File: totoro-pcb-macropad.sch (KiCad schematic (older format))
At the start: 37 parts, among them J1 USB4085-GF-A_REVA, SW1 SW_PUSH, U1 ATMEGA32U4, X1 XTAL_GND

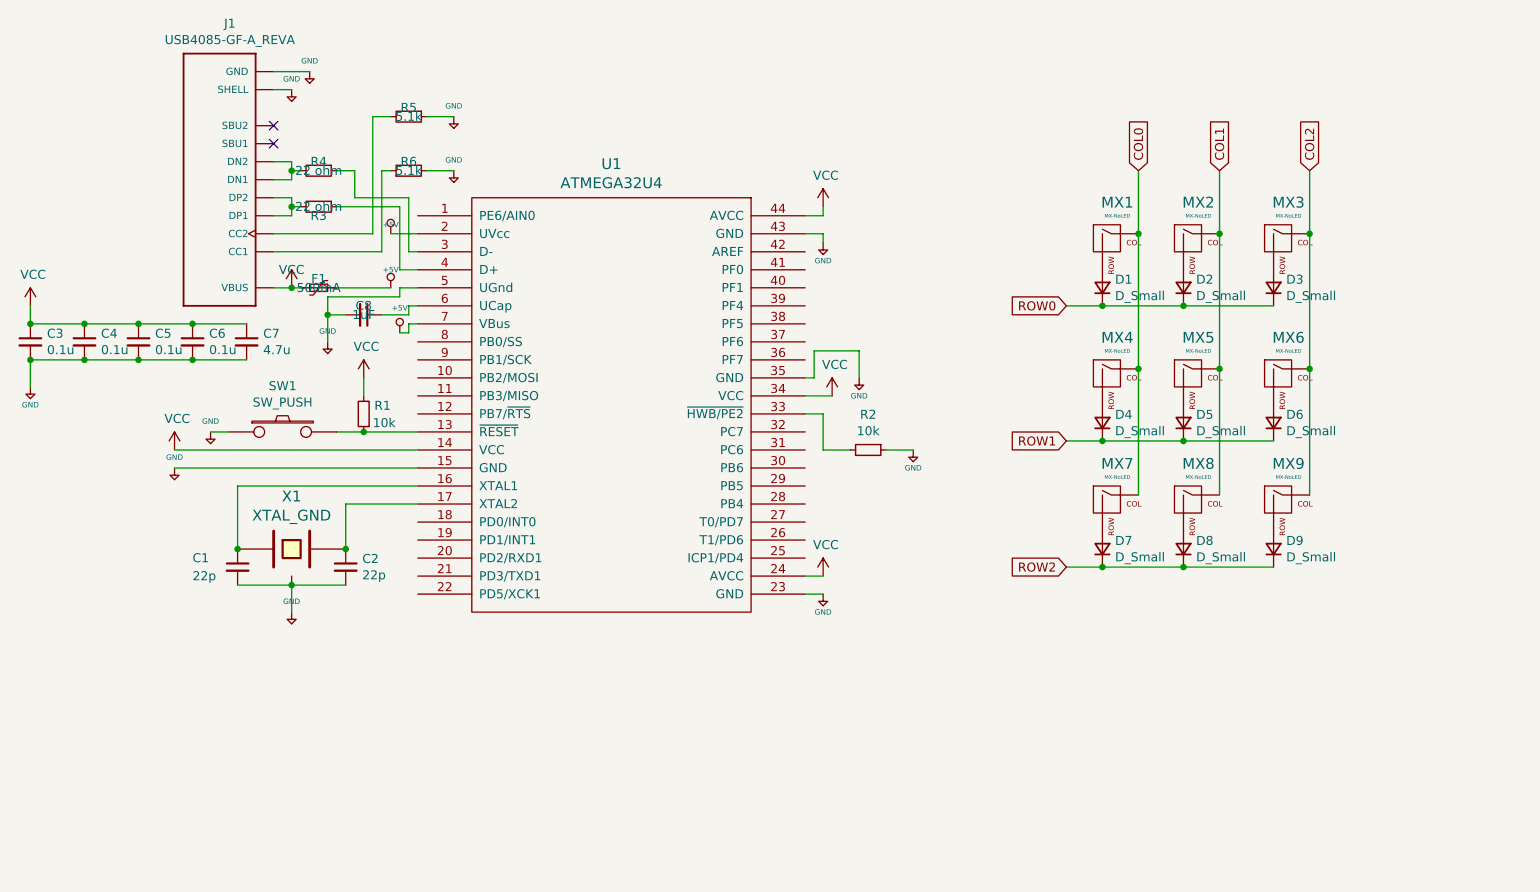
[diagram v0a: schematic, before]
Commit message: PCB layout
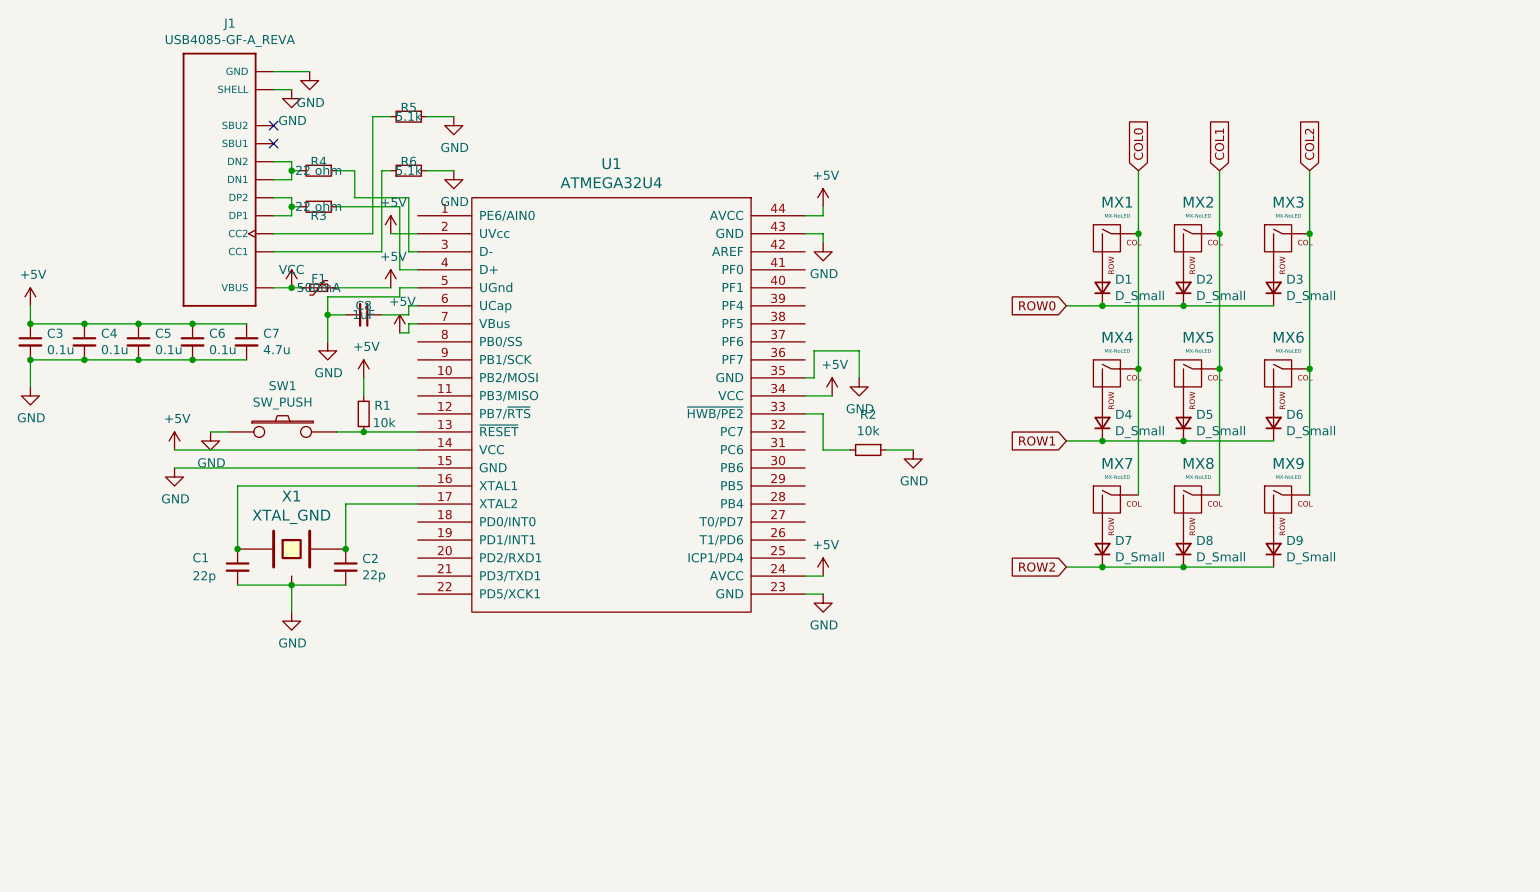
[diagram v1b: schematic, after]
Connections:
- net +5V: now also C3.1, C4.1, C5.1, C6.1, C7.1, R1.2, U1.14 (VCC), U1.24 (AVCC), U1.34 (VCC), U1.44 (AVCC); no longer C1.2, C2.2, C3.2, C4.2, C5.2, C6.2, C7.2, C8.2, J1.A1 (GND), J1.A12 (GND), J1.B1 (GND), J1.B12 (GND), J1.P1 (SHELL), J1.P2 (SHELL), J1.P3 (SHELL), J1.P4 (SHELL), R2.1, R5.1, R6.2, SW1.1, U1.15 (GND), U1.23 (GND), U1.35 (GND), U1.43 (GND), U1.5 (UGnd), X1.3
- net VCC: no longer C3.1, C4.1, C5.1, C6.1, C7.1, R1.2, U1.14 (VCC), U1.24 (AVCC), U1.34 (VCC), U1.44 (AVCC)
- new net GND: C1.2, C2.2, C3.2, C4.2, C5.2, C6.2, C7.2, C8.2, J1.A1 (GND), J1.A12 (GND), J1.B1 (GND), J1.B12 (GND), J1.P1 (SHELL), J1.P2 (SHELL), J1.P3 (SHELL), J1.P4 (SHELL), R2.1, R5.1, R6.2, SW1.1, U1.15 (GND), U1.23 (GND), U1.35 (GND), U1.43 (GND), U1.5 (UGnd), X1.3

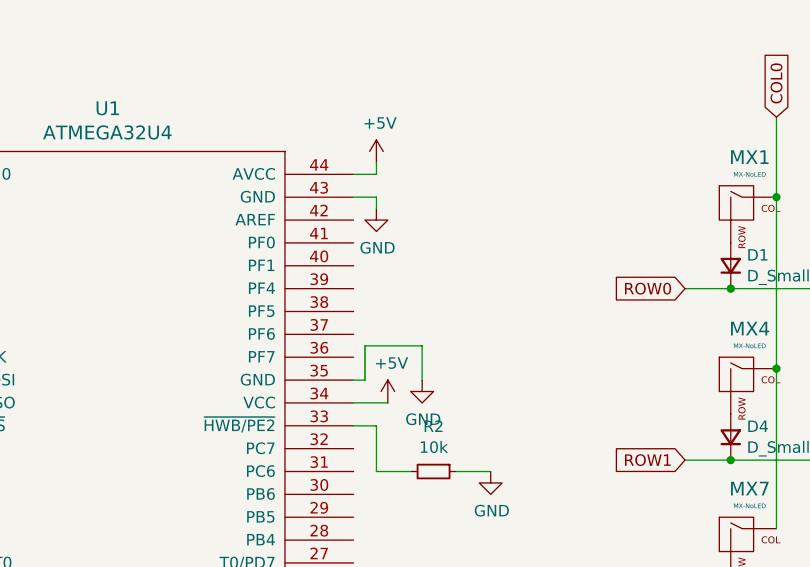
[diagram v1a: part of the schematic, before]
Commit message: Final commit
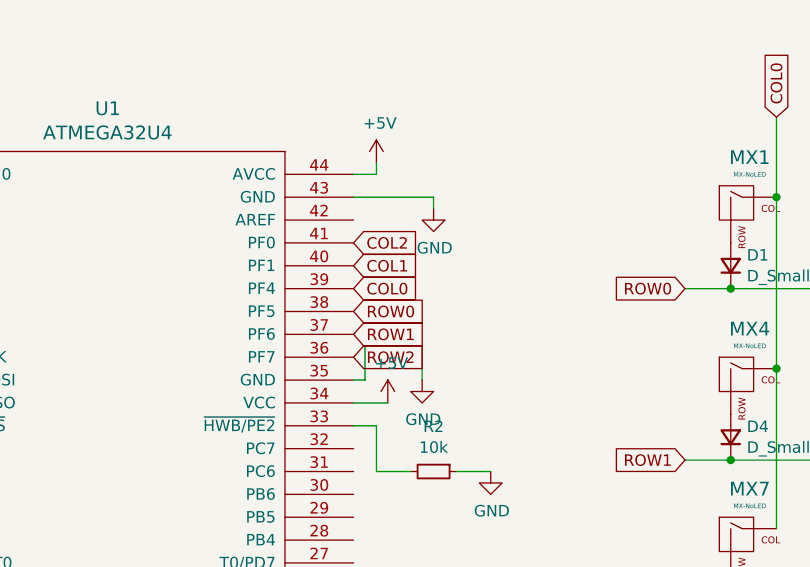
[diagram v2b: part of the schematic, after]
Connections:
- net COL0: now also U1.39 (PF4)
- net COL1: now also U1.40 (PF1)
- net COL2: now also U1.41 (PF0)
- net ROW0: now also U1.38 (PF5)
- net ROW1: now also U1.37 (PF6)
- net ROW2: now also U1.36 (PF7)
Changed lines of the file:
@@
 	2600 2250 2600 2400
-Wire Wire Line
-	5250 1800 5350 1800
-Wire Wire Line
-	5350 1800 5350 1850
 Wire Wire Line
 	5250 1700 5350 1700
@@
 L power:GND #PWR0105
 U 1 1 5F4F7593
-P 5350 1850
-F 0 "#PWR0105" H 5350 1600 50  0001 C CNN
-F 1 "GND" H 5355 1677 50  0000 C CNN
-F 2 "" H 5350 1850 50  0001 C CNN
-F 3 "" H 5350 1850 50  0001 C CNN
-	1    5350 1850
+P 5600 1850
+F 0 "#PWR0105" H 5600 1600 50  0001 C CNN
+F 1 "GND" H 5605 1677 50  0000 C CNN
+F 2 "" H 5600 1850 50  0001 C CNN
+F 3 "" H 5600 1850 50  0001 C CNN
+	1    5600 1850
 	1    0    0    -1
 $EndComp
@@
 	1    0    0    -1
 $EndComp
+Text GLabel 5250 2000 2    50   Input ~ 0
+COL2
+Wire Wire Line
+	5600 1800 5600 1850
+Wire Wire Line
+	5250 1800 5600 1800
+Text GLabel 5250 2100 2    50   Input ~ 0
+COL1
+Text GLabel 5250 2200 2    50   Input ~ 0
+COL0
+Text GLabel 5250 2300 2    50   Input ~ 0
+ROW0
+Text GLabel 5250 2400 2    50   Input ~ 0
+ROW1
+Text GLabel 5250 2500 2    50   Input ~ 0
+ROW2
 $EndSCHEMATC

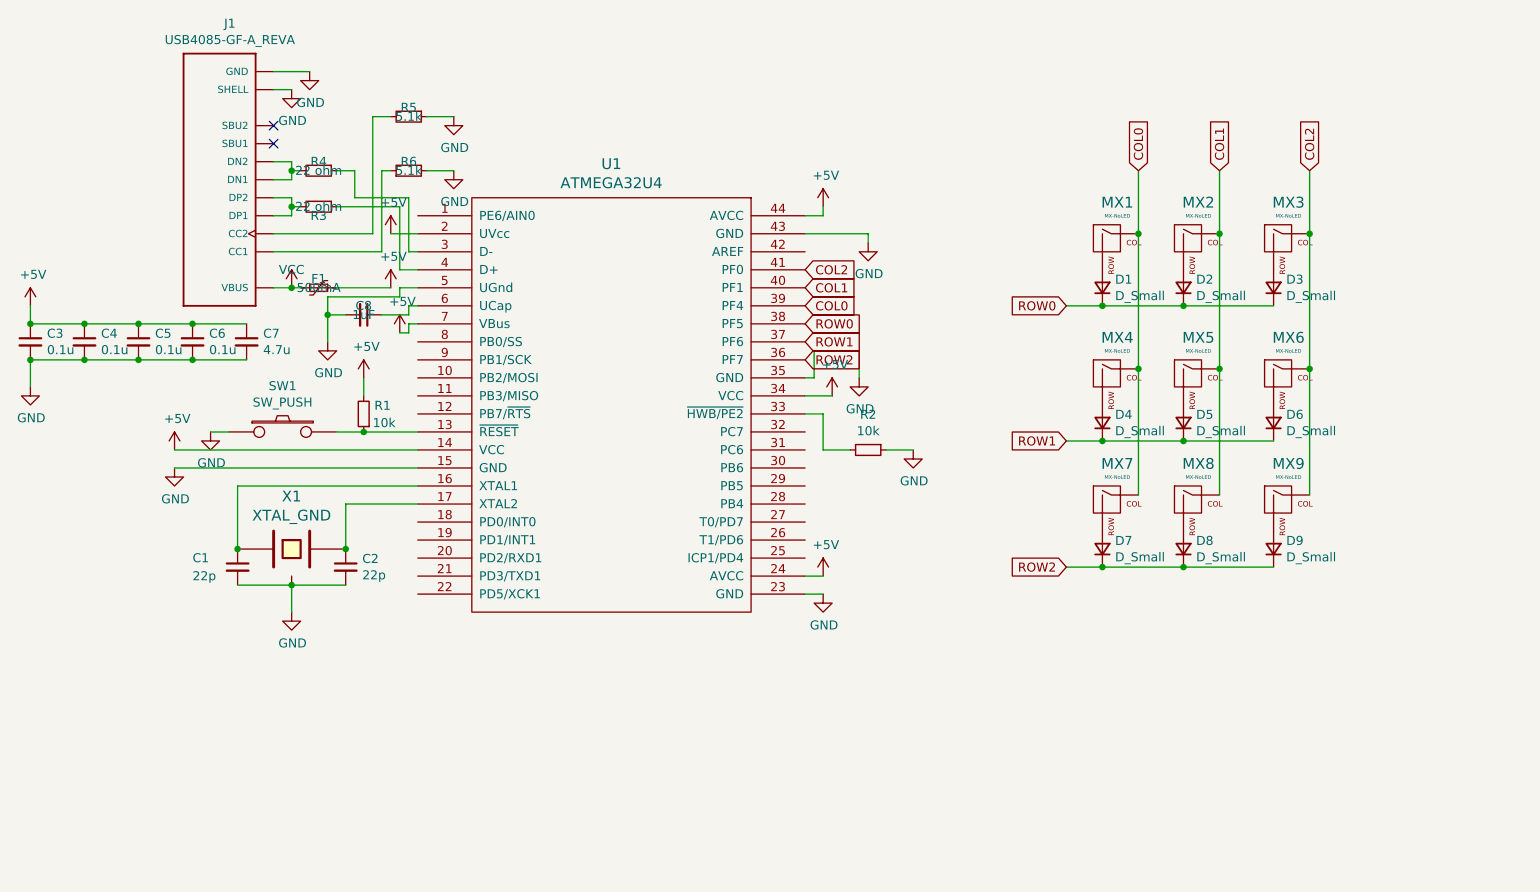
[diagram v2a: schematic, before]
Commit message: Probably fix crystal footprint, but i dont remember
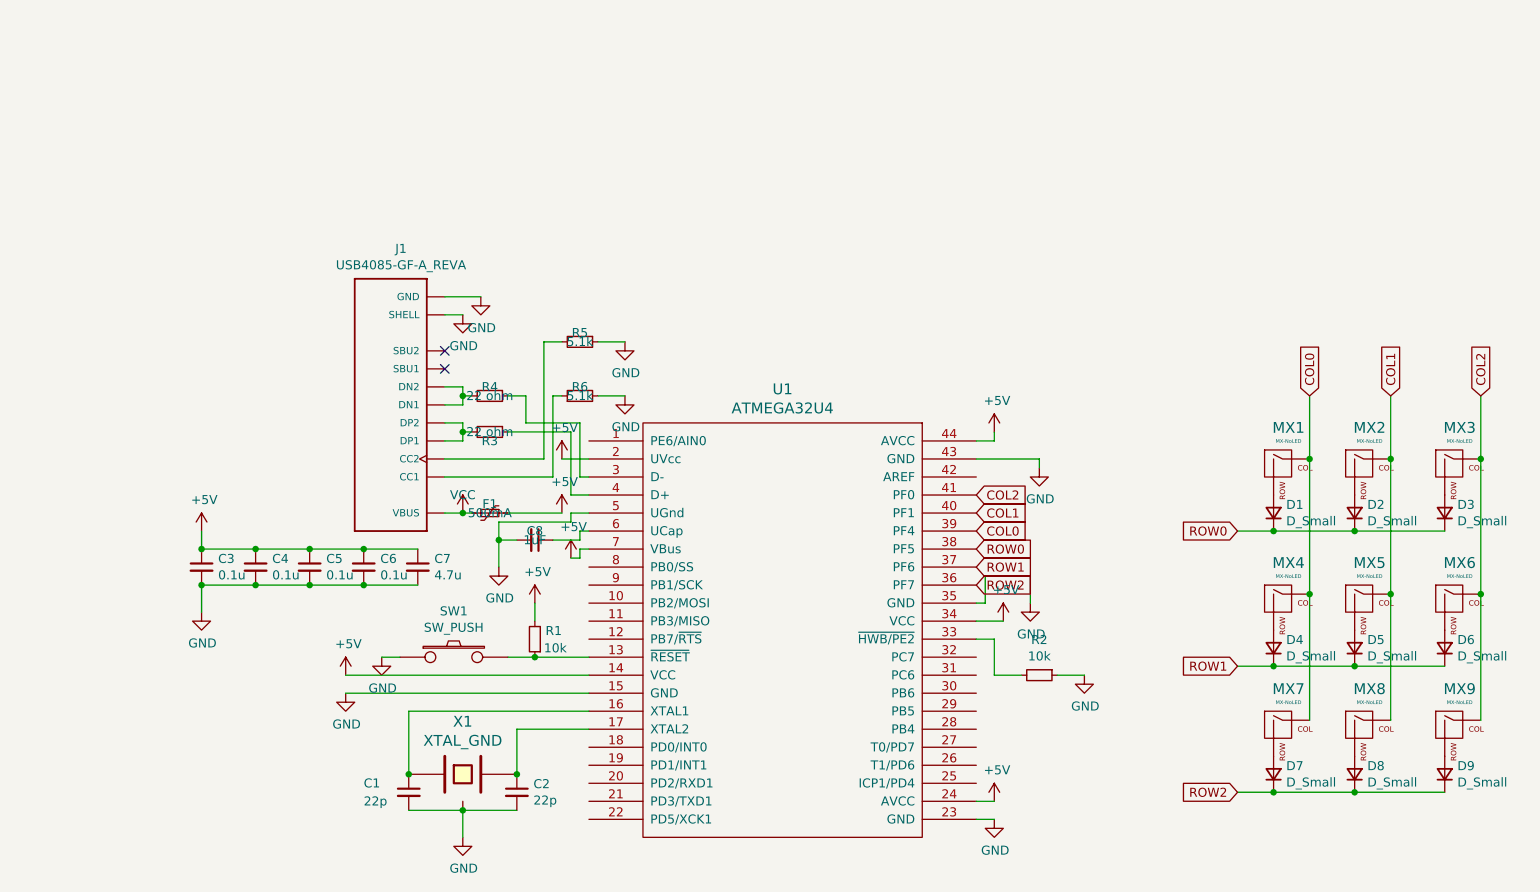
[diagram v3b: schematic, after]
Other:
- moved on the sheet: C1, C2, C3, C4, C5, C6, C7, C8, D1, D2, D3, D4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
